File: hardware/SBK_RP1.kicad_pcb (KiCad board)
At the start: 2 copper layers, 8.2 x 9.9 mm, 5 parts, among them J1 1 x 3 pin header, Q1 AO3401A

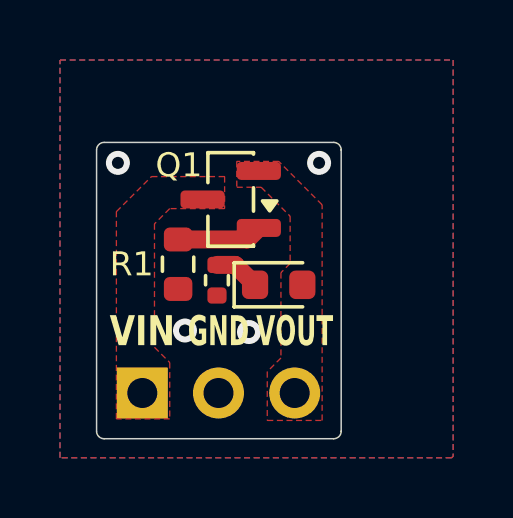
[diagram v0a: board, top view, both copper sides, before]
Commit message: images update
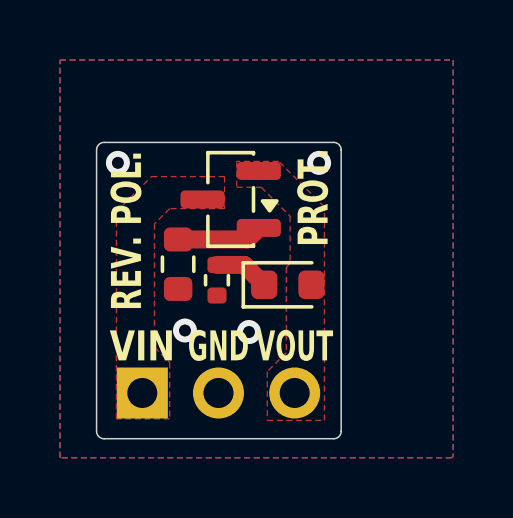
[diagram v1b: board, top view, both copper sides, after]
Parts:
- moved D1 0.30 mm to (119.2, 85.3)
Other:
- board text added: "PROT."
- board text added: "REV. POL."
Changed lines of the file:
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@@
 		(tags "SOT TO_SOT_SMD")
 		(property "Reference" "Q1"
-			(at 1.7272 1.143 0)
-			(layer "F.SilkS")
+			(at -2.54 0.1524 0)
+			(layer "F.SilkS")
+			(hide yes)
 			(effects
 				(font
@@
 		(property ki_fp_filters "SOT?23*")
 		(sheetname "/")
-		(sheetfile "SBK_RP1.kicad_sch")
-		(units
-			(unit
-				(name "A")
-				(pins "1" "3" "2")
-			)
-		)
+		(sheetfile "SBK_RP1_v1_0.kicad_sch")
 		(attr smd)
 		(duplicate_pad_numbers_are_jumpers no)
@@
 		)
 		(fp_line
-			(start 0.900001 1.7)
-			(end -0.900001 1.7)
+			(start 0.9 1.7)
+			(end -0.9 1.7)
 			(stroke
 				(width 0.05)
@@
 		)
 		(fp_line
-			(start 0.900001 -1.7)
-			(end 0.9 -0.55)
-			(stroke
-				(width 0.05)
-				(type solid)
-			)
-			(layer "F.CrtYd")
-		)
-		(fp_line
 			(start 0.9 0.55)
-			(end 0.900001 1.7)
+			(end 0.9 1.7)
 			(stroke
 				(width 0.05)
@@
 		)
 		(fp_line
+			(start 0.9 -1.7)
+			(end 0.9 -0.55)
+			(stroke
+				(width 0.05)
+				(type solid)
+			)
+			(layer "F.CrtYd")
+		)
+		(fp_line
+			(start -0.9 1.7)
+			(end -0.9 1.5)
+			(stroke
+				(width 0.05)
+				(type solid)
+			)
+			(layer "F.CrtYd")
+		)
+		(fp_line
 			(start -0.9 1.5)
 			(end -1.93 1.5)
@@
 		)
 		(fp_line
-			(start -0.9 0.390001)
-			(end -0.9 -0.390001)
+			(start -0.9 0.39)
+			(end -0.9 -0.39)
 			(stroke
 				(width 0.05)
@@
 		)
 		(fp_line
-			(start -0.9 -0.390001)
-			(end -1.93 -0.390001)
+			(start -0.9 -0.39)
+			(end -1.93 -0.39)
 			(stroke
 				(width 0.05)
@@
 		(fp_line
 			(start -0.9 -1.5)
-			(end -0.900001 -1.7)
+			(end -0.9 -1.7)
 			(stroke
 				(width 0.05)
@@
 		)
 		(fp_line
-			(start -0.900001 1.7)
-			(end -0.9 1.5)
+			(start -0.9 -1.7)
+			(end 0.9 -1.7)
 			(stroke
 				(width 0.05)
@@
 		)
 		(fp_line
-			(start -0.900001 -1.7)
-			(end 0.900001 -1.7)
+			(start -1.93 1.5)
+			(end -1.93 0.39)
 			(stroke
 				(width 0.05)
@@
 		)
 		(fp_line
-			(start -1.93 1.5)
-			(end -1.93 0.390001)
+			(start -1.93 0.39)
+			(end -0.9 0.39)
 			(stroke
 				(width 0.05)
@@
 		)
 		(fp_line
-			(start -1.93 0.390001)
-			(end -0.9 0.390001)
-			(stroke
-				(width 0.05)
-				(type solid)
-			)
-			(layer "F.CrtYd")
-		)
-		(fp_line
-			(start -1.93 -0.390001)
+			(start -1.93 -0.39)
 			(end -1.93 -1.5)
 			(stroke
@@
 		(fp_poly
 			(pts
-				(xy -0.325 -1.45) (xy 0.65 -1.45) (xy 0.65 1.45) (xy -0.65 1.45) (xy -0.65 -1.125001)
+				(xy -0.325 -1.45) (xy 0.65 -1.45) (xy 0.65 1.45) (xy -0.65 1.45) (xy -0.65 -1.125)
 			)
 			(stroke
@@
 		)
 		(pad "3" smd roundrect
-			(at 0.937501 0 180)
+			(at 0.9375 0 180)
 			(size 1.475 0.6)
 			(layers "F.Cu" "F.Mask" "F.Paste")
@@
 	(footprint "LED_SMD:LED_0603_1608Metric"
 		(layer "F.Cu")
-		(at 118.8466 85.2932)
+		(at 119.1514 85.2932)
 		(descr "LED SMD 0603 (1608 Metric), square (rectangular) end terminal, IPC-7351 nominal, (Body size source: http://www.tortai-tech.com/upload/download/2011102023233369053.pdf)")
 		(tags "LED")
@@
 		(property ki_fp_filters "LED* LED_SMD:* LED_THT:*")
 		(sheetname "/")
-		(sheetfile "SBK_RP1.kicad_sch")
+		(sheetfile "SBK_RP1_v1_0.kicad_sch")
 		(units
 			(unit
@@
 		(tags "resistor")
 		(property "Reference" "R1"
-			(at 0 1.5494 0)
-			(layer "F.SilkS")
+			(at 0.6604 1.397 0)
+			(layer "F.SilkS")
+			(hide yes)
 			(effects
 				(font
@@
 			)
 		)
-		(property "Description" "Gate series resistor"
+		(property "Description" "Gate protection resistor"
 			(at 0 0 90)
 			(layer "F.Fab")
@@
 		(property ki_fp_filters "R_*")
 		(sheetname "/")
-		(sheetfile "SBK_RP1.kicad_sch")
+		(sheetfile "SBK_RP1_v1_0.kicad_sch")
 		(units
 			(unit
@@
 		(property ki_fp_filters "R_*")
 		(sheetname "/")
-		(sheetfile "SBK_RP1.kicad_sch")
+		(sheetfile "SBK_RP1_v1_0.kicad_sch")
 		(units
 			(unit
@@
 		(property ki_fp_filters "Connector*:*_1x??_*")
 		(sheetname "/")
-		(sheetfile "SBK_RP1.kicad_sch")
-		(units
-			(unit
-				(name "A")
-				(pins "1" "2" "3")
-			)
-		)
+		(sheetfile "SBK_RP1_v1_0.kicad_sch")
 		(attr through_hole)
 		(duplicate_pad_numbers_are_jumpers no)
 		(fp_line
 			(start -1.38 1.38)
-			(end 0 1.379999)
+			(end 0 1.38)
 			(stroke
 				(width 0.12)
@@
 		)
 		(fp_line
-			(start -1.379999 0)
+			(start -1.38 0)
 			(end -1.38 1.38)
 			(stroke
@@
 			(layer "B.SilkS")
 		)
-		(fp_poly
-			(pts
-				(xy -1.77 1.77) (xy 1.77 1.77) (xy 1.77 -6.849999) (xy -1.77 -6.849999)
-			)
+		(fp_rect
+			(start -1.77 1.77)
+			(end 1.77 -6.85)
 			(stroke
 				(width 0.05)
@@
 		(fp_line
 			(start 1.27 1.27)
-			(end 1.270001 -6.35)
+			(end 1.27 -6.35)
 			(stroke
 				(width 0.1)
@@
 		)
 		(fp_line
-			(start -1.270001 -6.35)
+			(start -1.27 -6.35)
 			(end -1.27 0.635)
 			(stroke
@@
 		)
 		(fp_line
-			(start 1.270001 -6.35)
-			(end -1.270001 -6.35)
+			(start 1.27 -6.35)
+			(end -1.27 -6.35)
 			(stroke
 				(width 0.1)
@@
 		)
 		(pad "3" thru_hole circle
-			(at 0 -5.079999 270)
+			(at 0 -5.08 270)
 			(size 1.7 1.7)
 			(drill 1)
@@
 	)
 	(gr_text "GND"
-		(at 116.839 86.8426 0)
+		(at 116.839 87.3506 0)
 		(layer "F.SilkS")
 		(effects
@@
 	)
 	(gr_text "VOUT"
-		(at 119.379 86.8426 0)
+		(at 119.379 87.3506 0)
 		(layer "F.SilkS")
 		(effects
@@
 		)
 	)
+	(gr_text "REV. POL."
+		(at 113.792 86.156533 90)
+		(layer "F.SilkS")
+		(effects
+			(font
+				(size 1 0.7)
+				(thickness 0.14)
+				(bold yes)
+			)
+			(justify left)
+		)
+	)
+	(gr_text "PROT."
+		(at 120.015 84.0232 90)
+		(layer "F.SilkS")
+		(effects
+			(font
+				(size 1 0.7)
+				(thickness 0.14)
+				(bold yes)
+			)
+			(justify left)
+		)
+	)
 	(gr_text "VIN"
-		(at 114.299 86.8426 0)
+		(at 114.299 87.3506 0)
 		(layer "F.SilkS")
 		(effects
@@
 	)
 	(segment
-		(start 117.396701 84.630801)
-		(end 118.0591 85.2932)
+		(start 116.7892 84.630801)
+		(end 117.701501 84.630801)
 		(width 0.6)
 		(layer "F.Cu")
@@
 	)
 	(segment
-		(start 116.7892 84.630801)
-		(end 117.396701 84.630801)
+		(start 117.701501 84.630801)
+		(end 118.3639 85.2932)
 		(width 0.6)
 		(layer "F.Cu")
@@
 		(polygon
 			(pts
-				(xy 118.4656 89.8144) (xy 120.2944 89.8144) (xy 120.2944 82.6262) (xy 118.8466 81.1784) (xy 117.4496 81.1784)
-				(xy 117.4496 82.042) (xy 118.2624 82.042) (xy 119.2276 83.0072) (xy 119.2276 84.582) (xy 118.9228 84.8868)
-				(xy 118.9228 87.7316) (xy 118.4656 88.1888)
-			)
-		)
+				(xy 118.4656 89.8144) (xy 120.3706 89.8144) (xy 120.3706 82.7024) (xy 118.8466 81.1784) (xy 117.4496 81.1784)
+				(xy 117.4496 82.042) (xy 118.2624 82.042) (xy 119.2276 83.0072) (xy 119.2276 84.582) (xy 119.1006 84.709)
+				(xy 119.1006 87.5538) (xy 118.4656 88.1888)
+			)
+		)
